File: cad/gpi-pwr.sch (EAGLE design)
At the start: 89 parts, among them CN1 HEADER-1X2, CN2 HEADER-3X1, CN3 HEADER-1X2.4, Q1 MOSFETTO247REV, Q3 MOSFETTO247REV, Q5 MOSFETTO247REV, Q6 MOSFETTO247REV, Q7 MOSFETTO247REV, Q8 MOSFETTO247REV, U1 ACS709, U2 ACS709, U3 ACPL-P346P346, U4 ACPL-P346P346, U5 ACPL-P346P346, U6 ACPL-P346P346, U7 ACPL-P346P346, U8 ACPL-P346P346

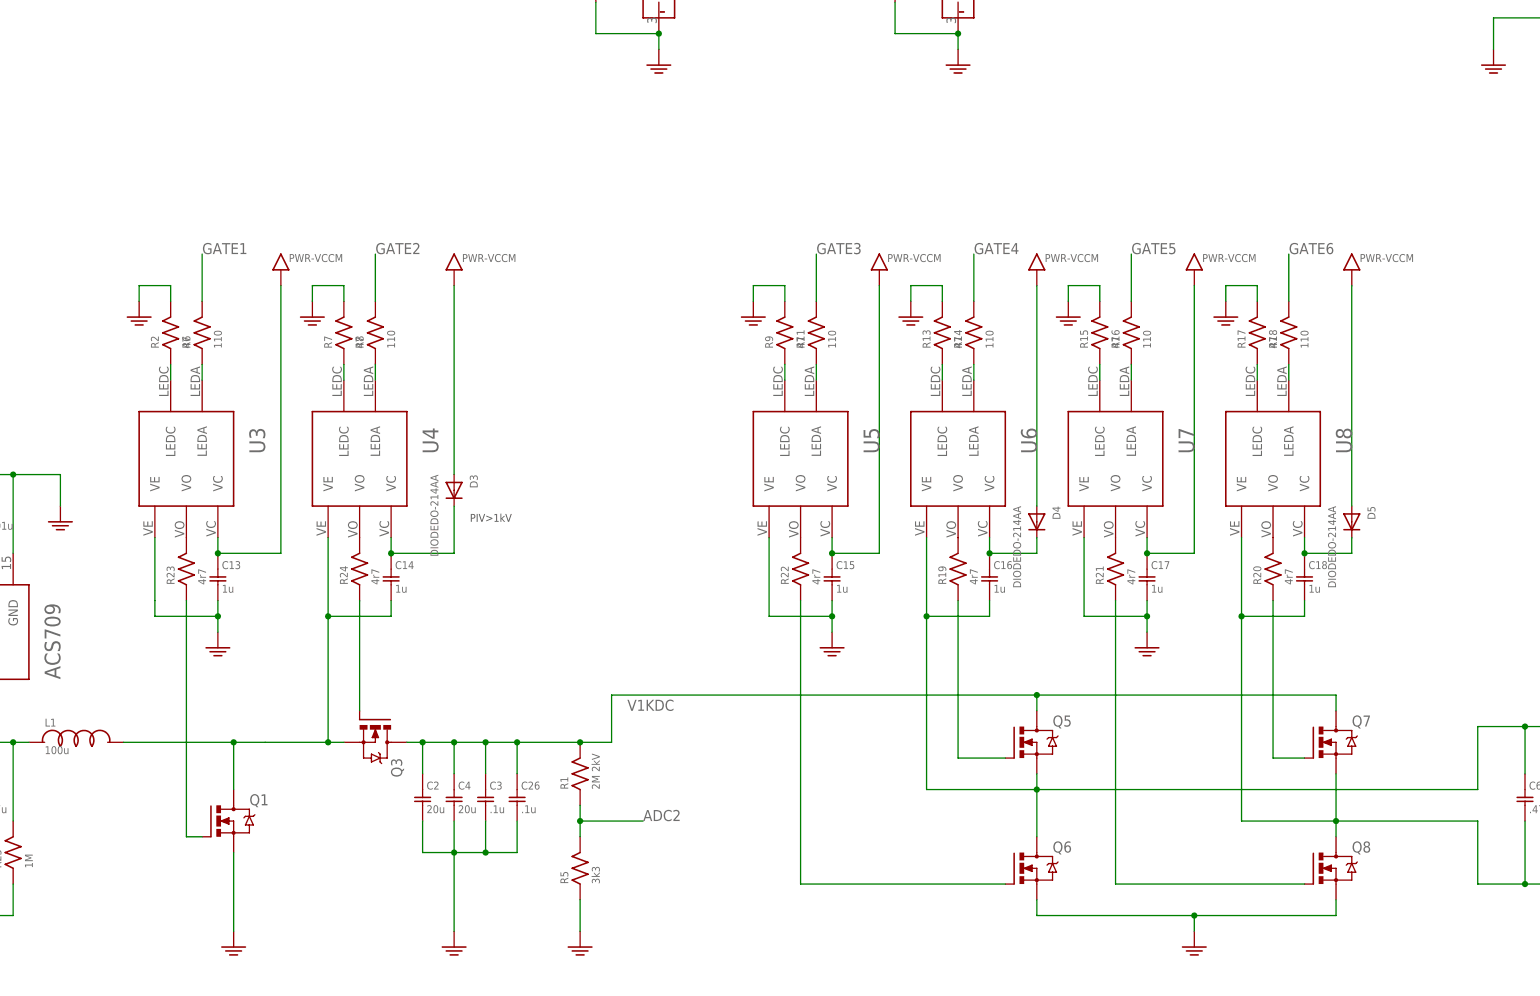
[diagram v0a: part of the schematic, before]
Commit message: gate snubbers
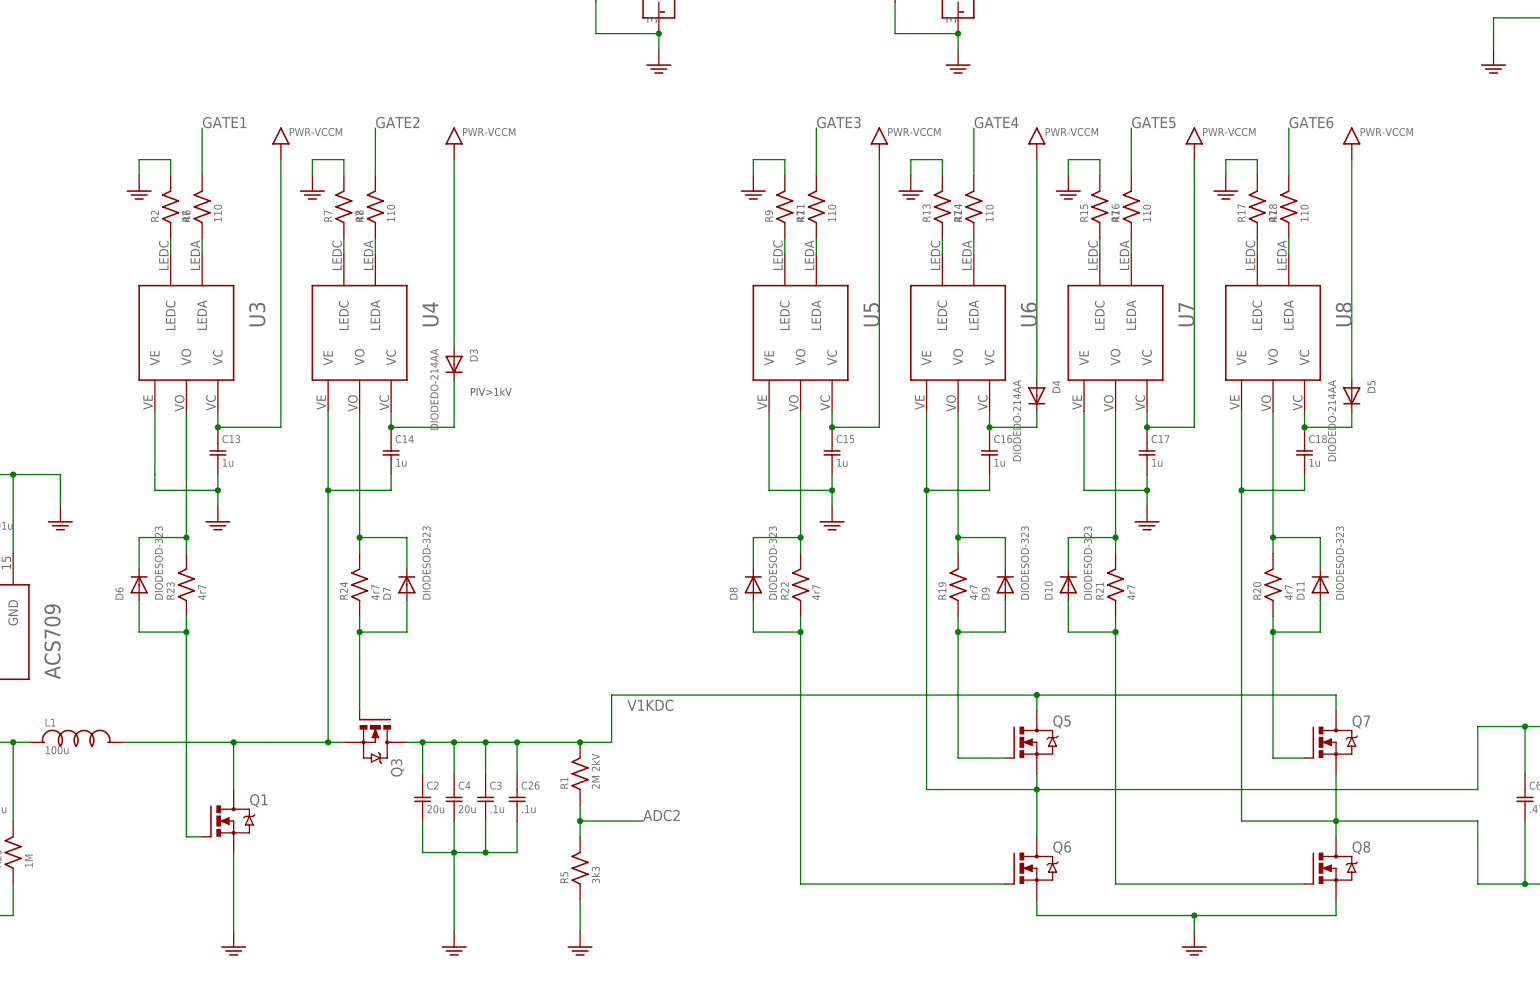
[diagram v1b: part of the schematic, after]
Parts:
- added D10, D11, D6, D7, D8, D9: DIODESOD-323, jaw:DIODESOD-323
- R19, R20, R21, R22, R23, R24: device jaw:R0612 -> jaw:RSMD0508
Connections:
- net N$19: now also D9.A
- net N$2: now also D9.C
- net N$20: now also D8.A
- net N$21: now also D10.A
- net N$22: now also D11.A
- net N$43: now also D11.C
- net N$44: now also D8.C
- net N$46: now also D10.C
- net N$47: now also D7.C
- net N$48: now also D7.A
- net N$5: now also D6.A
- net N$6: now also D6.C
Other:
- moved on the sheet: C13, C14, C15, C16, C17, C18, D3, D4, D5, R11, R13, R14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
